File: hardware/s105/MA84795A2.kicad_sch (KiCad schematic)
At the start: 9 parts, among them U4 case only

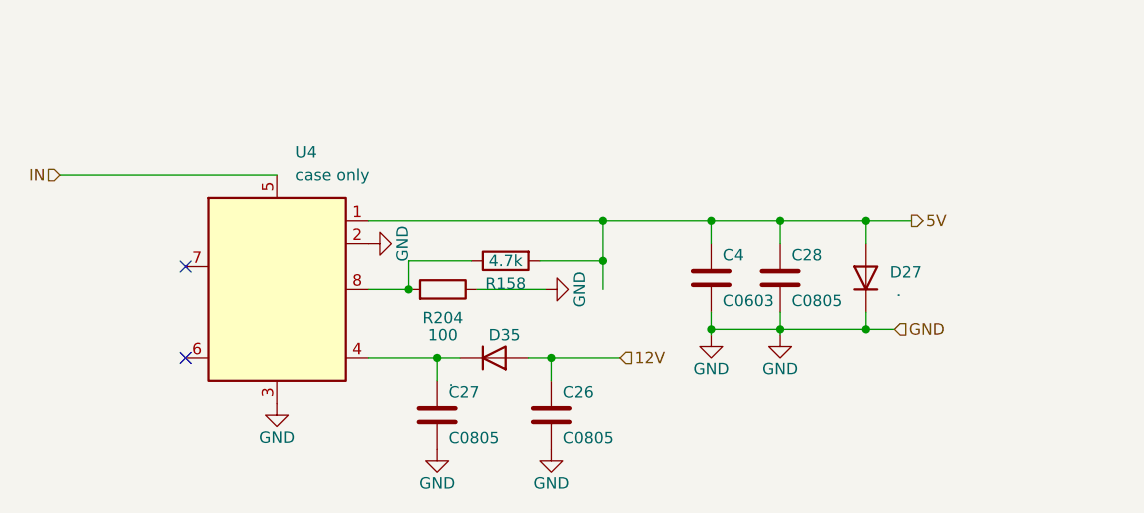
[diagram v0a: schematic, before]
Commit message: закончила пока что
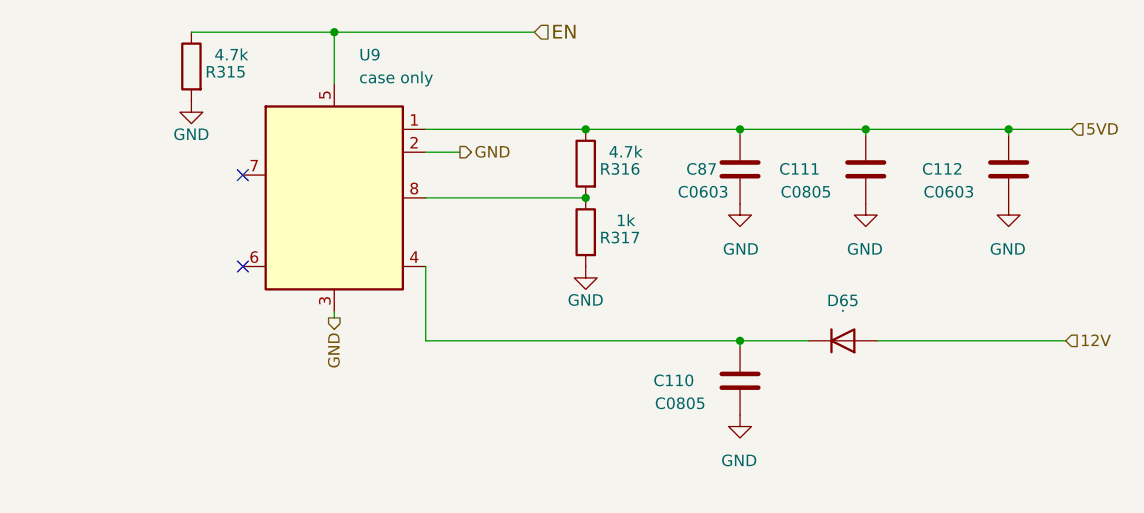
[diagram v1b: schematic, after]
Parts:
- removed C26, C27, C28: C0805, Capacitor_SMD:C_0805_2012Metric, symbol Device:C
- removed C4: C0603, Capacitor_SMD:C_0603_1608Metric, symbol Device:C
- removed D27: ., Diode_SMD:D_SMA, symbol Diode:US2JA
- removed D35: ., Diode_SMD:D_SOD-123, symbol Diode:1N4148W
- removed R158: 4.7k, Resistor_SMD:R_0603_1608Metric, symbol Device:R
- removed R204: 100, Resistor_SMD:R_0603_1608Metric, symbol Device:R
- removed U4: case only, Package_SO:SOIC-8_3.9x4.9mm_P1.27mm, symbol Regulator_Controller:L6727
- added C110, C111: C0805, Capacitor_SMD:C_0805_2012Metric, symbol Device:C
- added C112, C87: C0603, Capacitor_SMD:C_0603_1608Metric, symbol Device:C
- added D65: ., Diode_SMD:D_SMA, symbol Diode:US2JA
- added R315, R316: 4.7k, Resistor_SMD:R_0603_1608Metric, symbol Device:R
- added R317: 1k, Resistor_SMD:R_0603_1608Metric, symbol Device:R
- added U9: case only, Package_SO:SOIC-8_3.9x4.9mm_P1.27mm, symbol Regulator_Controller:L6727
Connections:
- net 12V: now also D65.2 (A)
- net GND: now also C110.2, C111.2, C112.2, C87.2, R315.2, R317.2, U9.2 (UGATE), U9.3 (GND)
- new net: R316.2, R317.1, U9.8 (PHASE)
- new net: C110.1, D65.1 (K), U9.4 (LGATE)
- new net 5VD: C111.1, C112.1, C87.1, R316.1, U9.1 (BOOT)
- new net EN: R315.1, U9.5 (VCC)

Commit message: #4 #5 #6 #8
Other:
- company: (none) -> rusEFI
- title: (none) -> s105
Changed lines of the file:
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@@
 (kicad_sch (version 20211123) (generator eeschema)
-  (paper "A4")
+  (paper "A3" portrait)
+  (title_block
+    (title "s105")
+    (rev "0.1")
+    (company "rusEFI")
+  )
   (junction (at 135.255 66.04) (diameter 0) (color 0 0 0 0)
   )
